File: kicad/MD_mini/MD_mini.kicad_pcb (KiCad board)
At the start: 2 copper layers, 58.6 x 36.3 mm, 65 parts, among them J1 Conn_01x02_Pin, J2 Conn_01x03_Pin, J3 Conn_01x02_Pin, J4 Conn_01x02_Pin, J6 Conn_02x03_Odd_Even, U1 IRS2003, U2 SCM3723ASA, U3 IRS2003, U4 ACS711xEXLT-15AB, U7 IRS2003, U8 IRS2003, U9 SCM3723ASA

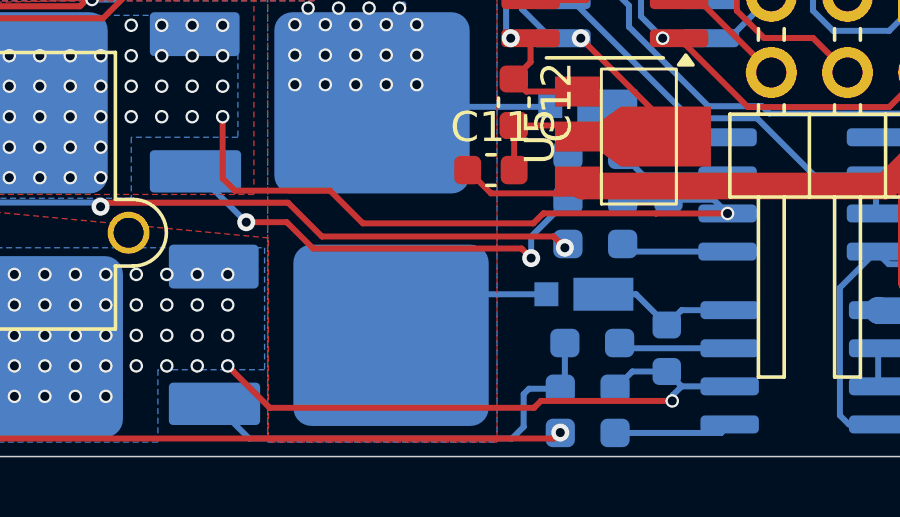
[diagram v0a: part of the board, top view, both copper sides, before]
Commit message: a
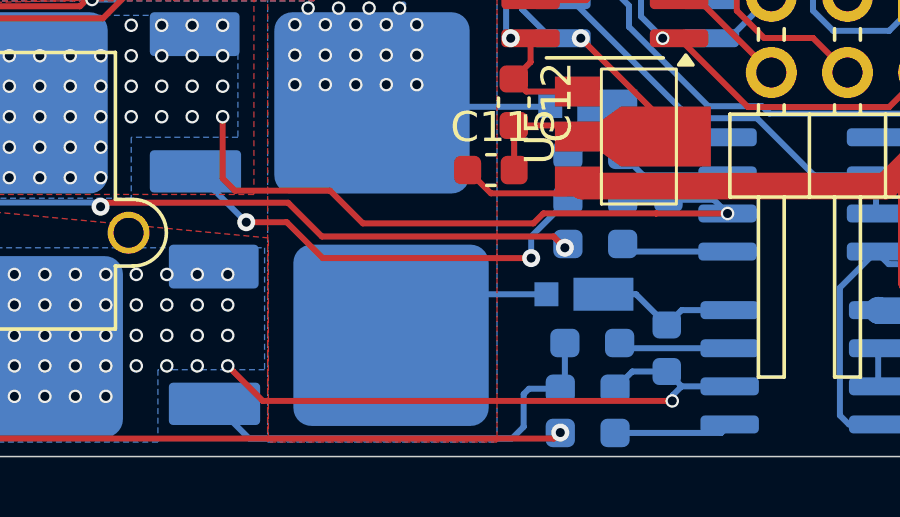
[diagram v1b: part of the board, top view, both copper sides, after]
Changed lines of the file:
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@@
 	)
 	(segment
-		(start 173.27 129.032)
+		(start 173.0414 128.8034)
 		(end 171.873 127.635)
 		(width 0.2)
@@
 	)
 	(segment
-		(start 182.084 129.032)
-		(end 173.27 129.032)
-		(width 0.2)
-		(layer "F.Cu")
-		(net 5)
-	)
-	(segment
-		(start 182.3126 128.8034)
-		(end 182.084 129.032)
-		(width 0.2)
-		(layer "F.Cu")
-		(net 5)
-	)
-	(segment
 		(start 186.69 128.8034)
-		(end 182.3126 128.8034)
+		(end 173.0414 128.8034)
 		(width 0.2)
 		(layer "F.Cu")
@@
 	)
 	(segment
-		(start 181.6682 123.7234)
-		(end 181.987165 124.042365)
+		(start 173.840665 122.845765)
+		(end 172.490065 122.845765)
 		(width 0.2)
 		(layer "F.Cu")
@@
 	)
 	(segment
-		(start 173.840665 122.845765)
-		(end 174.7183 123.7234)
+		(start 175.037265 124.042365)
+		(end 173.840665 122.845765)
 		(width 0.2)
 		(layer "F.Cu")
@@
 	)
 	(segment
-		(start 172.490065 122.845765)
-		(end 173.840665 122.845765)
-		(width 0.2)
-		(layer "F.Cu")
-		(net 17)
-	)
-	(segment
-		(start 174.7183 123.7234)
-		(end 181.6682 123.7234)
-		(width 0.2)
-		(layer "F.Cu")
+		(start 181.987165 124.042365)
+		(end 175.037265 124.042365)
+		(width 0.2)
+		(layer "F.Cu")

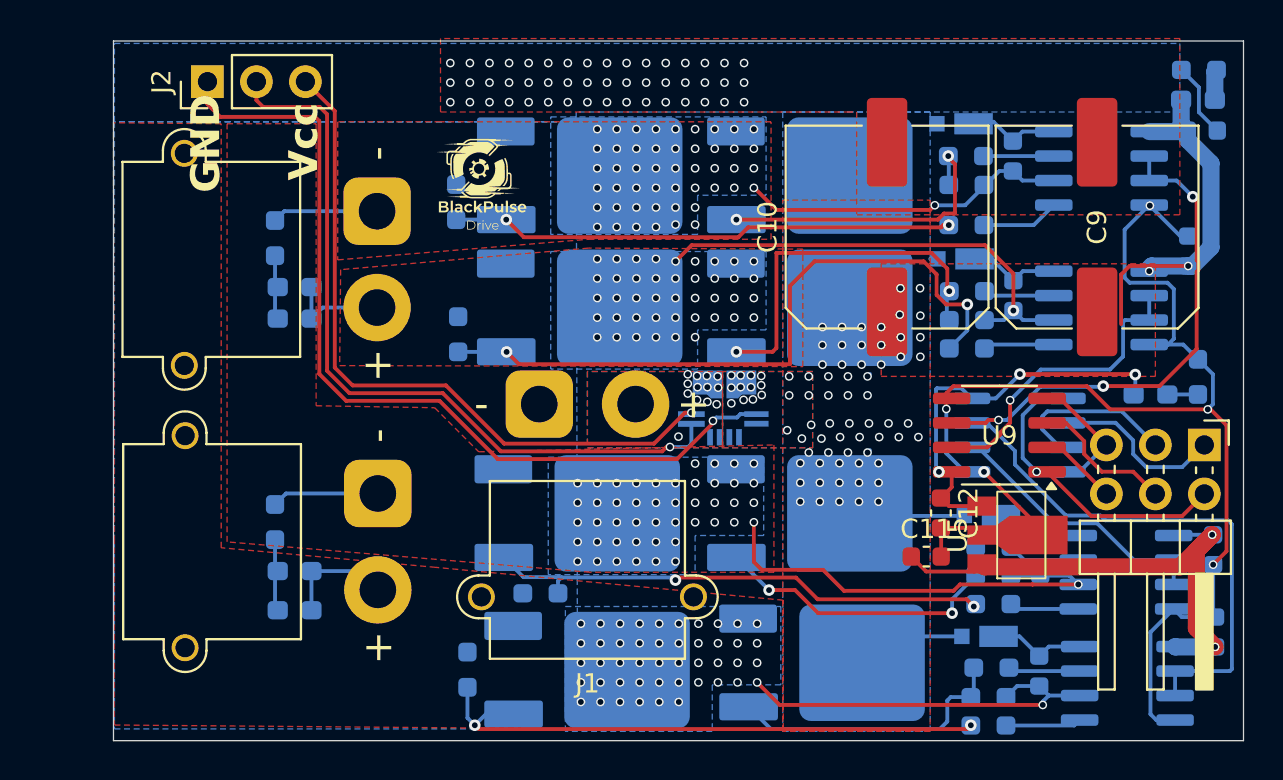
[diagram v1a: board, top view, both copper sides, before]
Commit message: a
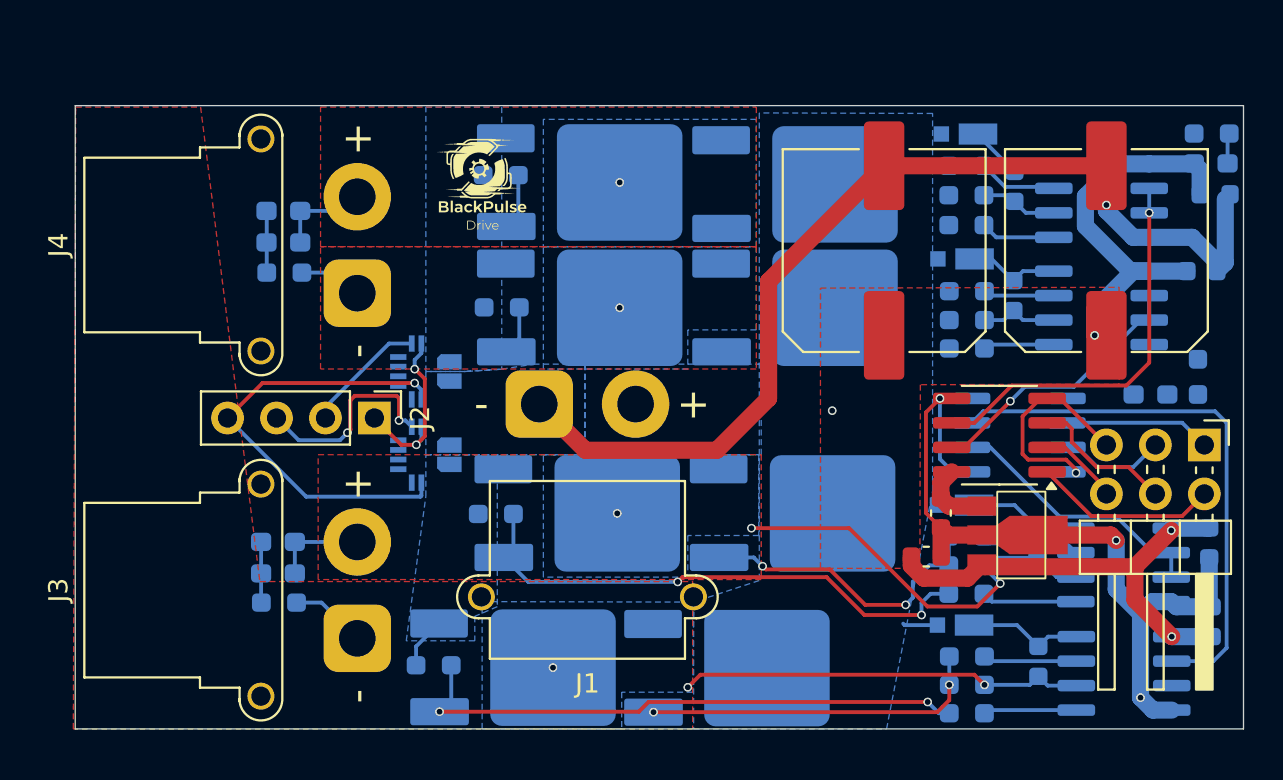
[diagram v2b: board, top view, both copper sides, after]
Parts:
- added U6: ACS711xEXLT-15AB, Sensor_Current:Allegro_QFN-12-10-1EP_3x3mm_P0.5mm, B.Cu at (154.7, 115.8)
- J2: value Conn_01x03_Pin -> Conn_01x04_Pin; footprint Connector_PinHeader_2.54mm:PinHeader_1x03_P2.54mm_Vertical -> Connector_PinHeader_2.54mm:PinHeader_1x04_P2.54mm_Vertical
- J3, J4: footprint Connector_AMASS:AMASS_XT30PW-M_1x02_P2.50mm_Horizontal -> Connector_AMASS:AMASS_XT30PW-F_1x02_P2.50mm_Horizontal
- R3, R4: value 10 -> 10k
- moved J2 19.5 mm to (152.0, 113.9), turned to -90 degrees
- moved U4 15.6 mm to (154.7, 111.5), turned to 180 degrees
- moved J3 7.59 mm to (151.1, 125.3)
- moved Q3 4.94 mm to (168.9, 126.9)
- moved R18 4.72 mm to (158.3, 118.9)
- moved J4 4.37 mm to (151.1, 107.4)
- moved R14 4.18 mm to (147.1, 123.5), turned to 180 degrees
- moved D5 3.99 mm to (147.3, 103.2)
- moved D6 3.99 mm to (147.3, 104.8)
- moved Q4 3.84 mm to (157.8, 126.8)
- moved R20 3.37 mm to (195.5, 99.2)
- moved C7 3.37 mm to (195.6, 102.3)
- moved D9 3.37 mm to (195.4, 100.7)
- moved R3 2.70 mm to (158.6, 101.3), turned to 0 degrees
- moved R7 2.66 mm to (158.6, 108.2), turned to 0 degrees
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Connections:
- net Net-(J2-Pin_2) renamed cur_1
- D5 pad 1: ch1_2 -> ch1_1
- D6 pad 2: ch1_2 -> ch1_1
- D7 pad 2: ch2_2 -> ch2_1
- D8 pad 1: ch2_2 -> ch2_1
- J1 pad 2: Net-(J1-Pin_2) -> VCC
- J2 pad 1: Net-(J2-Pin_1) -> VDDA
- J2 pad 3: Net-(J2-Pin_3) -> cur_2
- J3 pad 1: ch2_1 -> ch2_2
- J3 pad 2: ch2_2 -> ch2_1
- J4 pad 1: ch1_1 -> ch1_2
- J4 pad 2: ch1_2 -> ch1_1
- Q2 pad 3: GND -> Net-(Q2-S)
- Q4 pad 3: GND -> Net-(Q4-S)
- Q6 pad 3: GND -> Net-(Q4-S)
- Q7 pad 3: GND -> Net-(Q2-S)
- R13 pad 1: ch1_1 -> ch1_2
- R14 pad 1: ch2_1 -> ch2_2
- R15 pad 1: GND -> Net-(Q4-S)
- R18 pad 1: GND -> Net-(Q4-S)
- R3 pad 1: GND -> Net-(Q2-S)
- R7 pad 1: GND -> Net-(Q2-S)
- U4 pad 1: Net-(J1-Pin_2) -> Net-(Q2-S)
- U4 pad 10: Net-(J2-Pin_3) -> VDDA
- U4 pad 2: VCC -> GND
- U4 pad 3: Net-(J2-Pin_1) -> GNDS
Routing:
- net Net-(J2-Pin_1): track 45.8 -> 0.00 mm, vias 1 -> 0
- net Net-(J2-Pin_3): track 36.3 -> 0.00 mm, vias 1 -> 0
- net cur_1: track 40.1 -> 6.41 mm, vias 1 -> 0
- net Net-(Q2-G): track 35.5 -> 2.59 mm, vias 2 -> 0
- net GNDS: track 0.00 -> 23.9 mm, vias 0 -> 1
- net Net-(Q7-G): track 26.2 -> 2.92 mm, vias 2 -> 0
- net ch1_2: track 29.7 -> 7.32 mm, vias 43 -> 1
- net Net-(Q1-G): track 19.1 -> 0.00 mm, vias 2 -> 0
- net GND: track 72.1 -> 89.1 mm, vias 53 -> 4
- net Net-(D10-A): track 20.4 -> 3.89 mm, vias 3 -> 0
- net Net-(Q8-G): track 16.1 -> 0.00 mm, vias 2 -> 0
- net ch1_1: track 22.6 -> 8.90 mm, vias 49 -> 1
- net VCC: track 59.6 -> 46.5 mm, vias 79 -> 4
- net cur_2: track 0.00 -> 10.7 mm, vias 0 -> 2
- net VDDA: track 0.00 -> 9.60 mm, vias 0 -> 2
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- added copper zone on B.Cu, net Net-(Q2-S)
- added copper zone on B.Cu, net Net-(Q4-S)
- removed copper zone on F.Cu, net GND
- removed copper zone on B.Cu, net Net-(J1-Pin_2)
- removed copper zone on F.Cu, net Net-(J1-Pin_2)
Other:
- board size 58.6 x 36.3 mm -> 60.6 x 32.3 mm
- board text removed: "GND"
- board text removed: "Vcc"
